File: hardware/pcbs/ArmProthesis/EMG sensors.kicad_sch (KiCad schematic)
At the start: 25 parts, among them IC1 INA128, U1 OPA2188AIDR, U4 OPA188AIDR

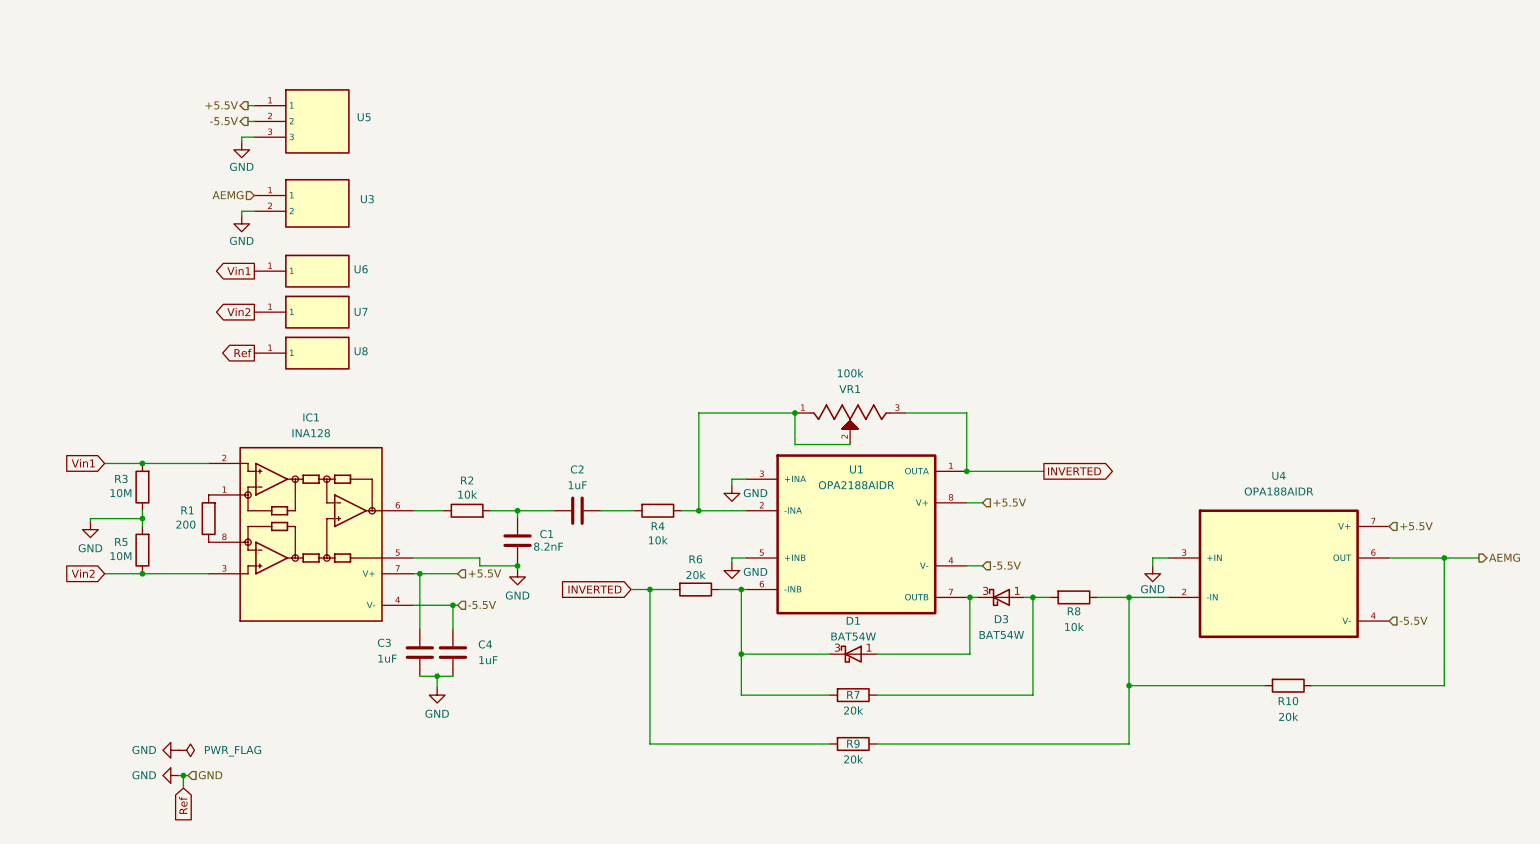
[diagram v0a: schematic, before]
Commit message: BMS v0.3 + main folder reconstruction
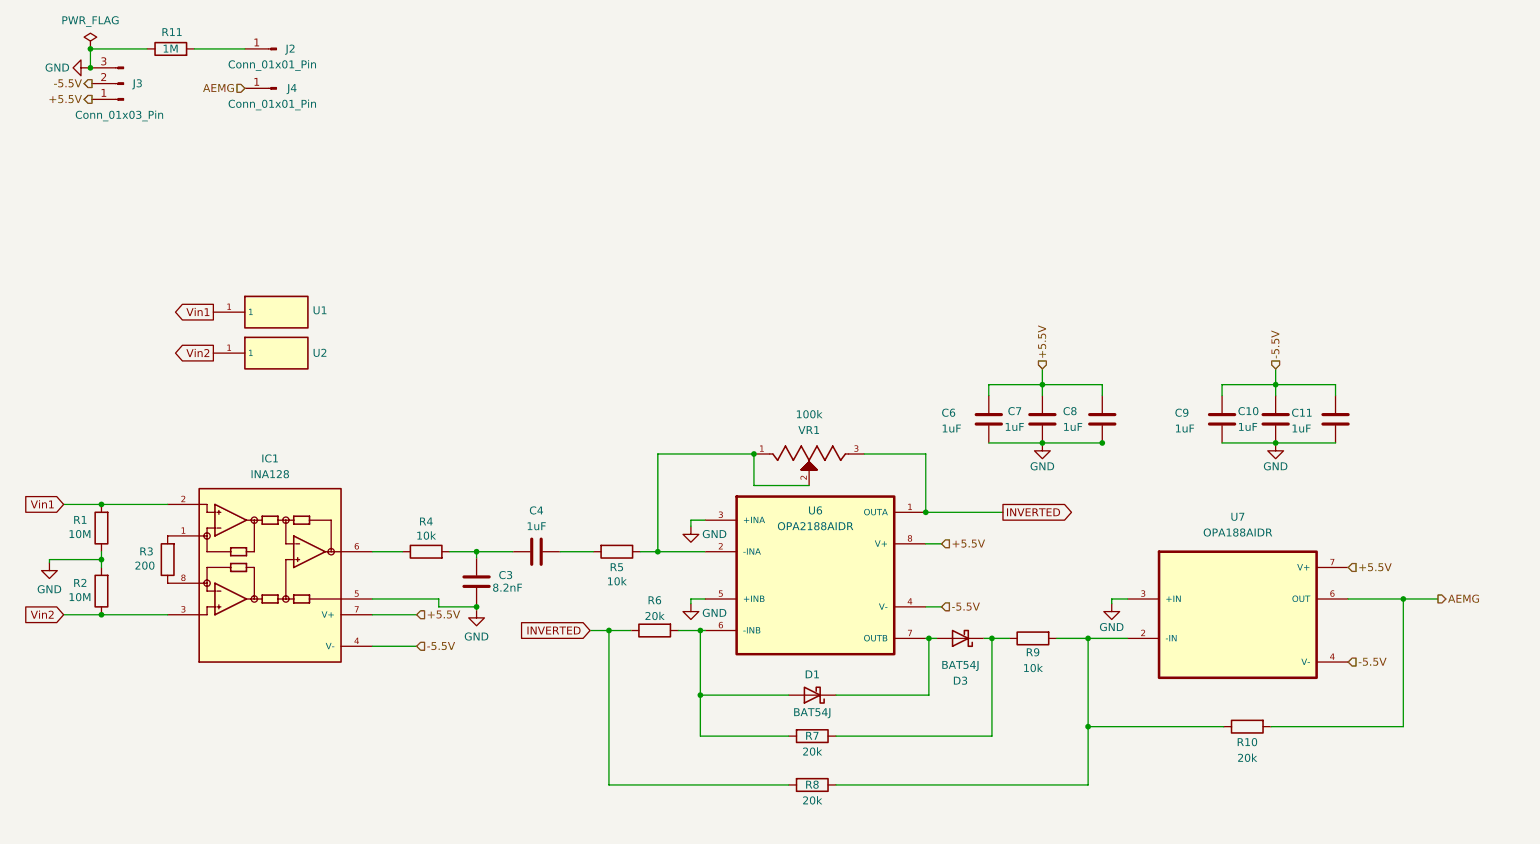
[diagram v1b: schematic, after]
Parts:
- removed C1: 8.2nF, Capacitor_SMD:C_0603_1608Metric_Pad1.08x0.95mm_HandSolder, symbol Device:C
- removed C2: 1uF, Capacitor_SMD:C_0603_1608Metric_Pad1.08x0.95mm_HandSolder, symbol Device:C
- removed D1, D3: BAT54W, Package_TO_SOT_SMD:SOT-323_SC-70, symbol Diode:BAT54W
- removed U1: OPA2188AIDR, OP AMPS:ОПА2188AIDR, symbol OP AMPS:OPA2188AIDR
- removed U3: ~, Connector_JST:JST_GH_BM02B-GHS-TBT_1x02-1MP_P1.25mm_Vertical, symbol headers:H_2
- removed U4: OPA188AIDR, OP AMPS:OPA188, symbol OP AMPS:OPA188AIDR
- removed U5: ~, Connector_JST:JST_GH_BM03B-GHS-TBT_1x03-1MP_P1.25mm_Vertical, symbol headers:H_3
- removed U6, U7, U8: ~, EMG:EMG_Snap_4mm, symbol headers:H_1
- added C10, C11, C6, C7, C8, C9: 1uF, Capacitor_SMD:C_0603_1608Metric_Pad1.08x0.95mm_HandSolder, symbol Device:C
- added D1, D3: BAT54J, Diode_SMD:D_SOD-323F, symbol Diode:BAT54J
- added J2, J4: Conn_01x01_Pin, Connectors:DIN_Male_1PIN_1.5mm, symbol Connector:Conn_01x01_Pin
- added J3: Conn_01x03_Pin, Connector_JST:JST_GH_SM03B-GHS-TB_1x03-1MP_P1.25mm_Horizontal, symbol Connector:Conn_01x03_Pin
- added R11: 1M, Resistor_SMD:R_0603_1608Metric_Pad0.98x0.95mm_HandSolder, symbol Device:R
- added U1, U2: ~, EMG:EMG_Snap_4mm, symbol headers:H_1
- added U6: OPA2188AIDR, OP AMPS:ОПА2188AIDR, symbol OP AMPS:OPA2188AIDR
- added U7: OPA188AIDR, OP AMPS:OPA188, symbol OP AMPS:OPA188AIDR
- C3: value 1uF -> 8.2nF; Website https://www.digikey.in/en/products/detail/kyocera-avx/KGM15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 -> https://eu.mouser.com/ProductDetail/KEMET/C0603X822F5JACTU?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
- IC1: footprint OP AMPS:INA128 -> OP AMPS:INA128U
- R1: value 200 -> 10M
- R2: value 10k -> 10M; Website (none) -> https://eu.mouser.com/ProductDetail/TE-Connectivity-Holswor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
- R3: value 10M -> 200
- R5: value 10M -> 10k; Website https://eu.mouser.com/ProductDetail/TE-Connectivity-Holswor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 -> (none)
- R8: value 10k -> 20k
- R9: value 20k -> 10k
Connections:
- net +5.5V: now also C6.1, C7.1, C8.1, J3.1 (Pin_1), U6.8 (V+), U7.7 (V+); no longer C3.1
- net -5.5V: now also C10.1, C11.1, C9.1, J3.2 (Pin_2), U6.4 (V-), U7.4 (V-); no longer C4.1
- net AEMG: now also R10.2, J4.1 (Pin_1), U7.6 (OUT); no longer R10.1
- net GND: now also R1.1, R2.2, C10.2, C11.2, C6.2, C7.2, C8.2, C9.2, J3.3 (Pin_3), R11.1, U6.3 (+INA), U6.5 (+INB), U7.3 (+IN); no longer C4.2, R3.1, R5.2
- net INVERTED: now also R6.1, R8.2, U6.1 (OUTA); no longer R6.2, R9.2
- net Vin1: now also R1.2, U1.1; no longer R3.2
- net Vin2: now also R2.1, U2.1; no longer R5.1
- net at R7.1: now also R9.1, D3.1 (K); no longer R8.2
- net at R7.2: now also R6.2, D1.2 (A), U6.6 (-INB); no longer R6.1
- net at IC1.1: now also R3.2; no longer R1.2
- net at IC1.6: now also R4.1; no longer R2.1
- net at IC1.8: now also R3.1; no longer R1.1
- net at R4.2: now also C3.1, C4.2
- net at VR1.1, VR1.2: now also R5.1, U6.2 (-INA); no longer R4.1
- new net: J2.1 (Pin_1), R11.2
- new net: D1.1 (K), D3.2 (A), U6.7 (OUTB)
- new net: R10.1, R8.1, R9.2, U7.2 (-IN)
- new net: C4.1, R5.2
